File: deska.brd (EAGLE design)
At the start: 50.5 x 49.5 mm, 7 parts

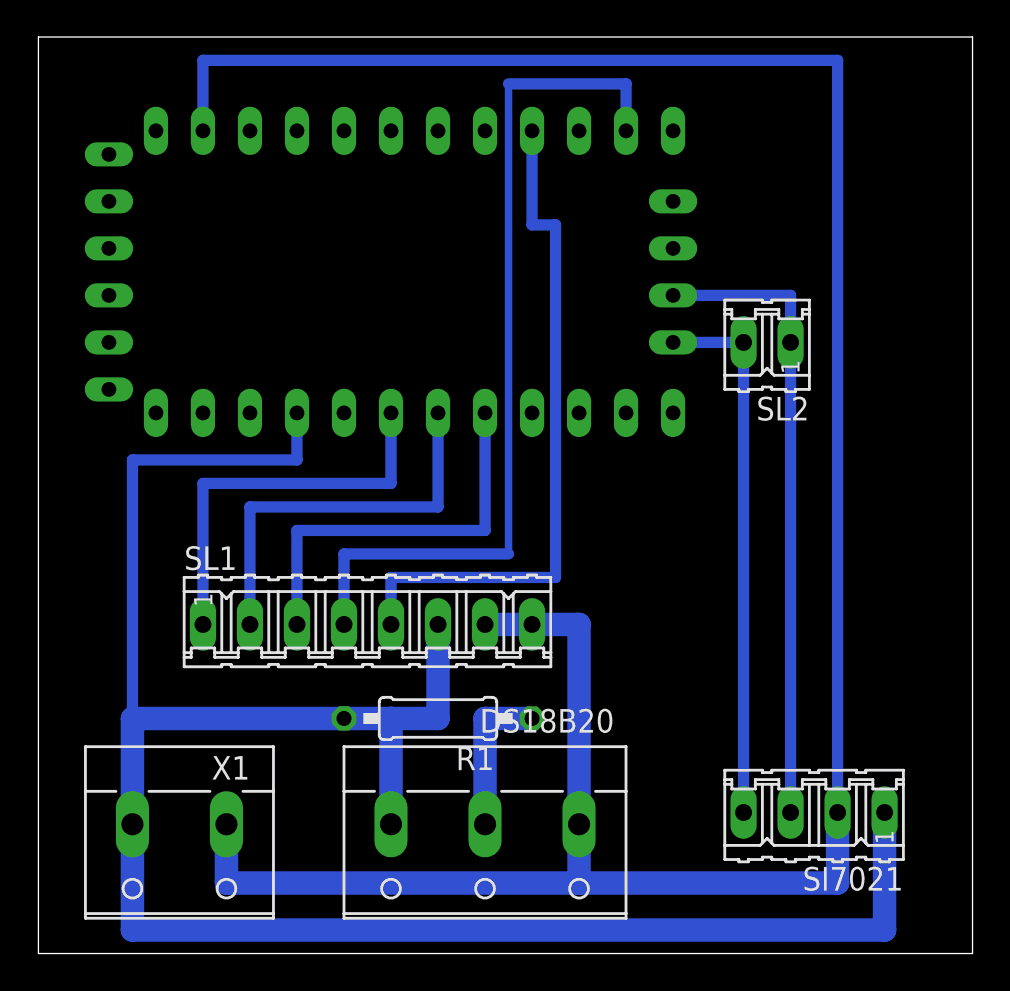
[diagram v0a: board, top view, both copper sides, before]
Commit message: +deska +ino
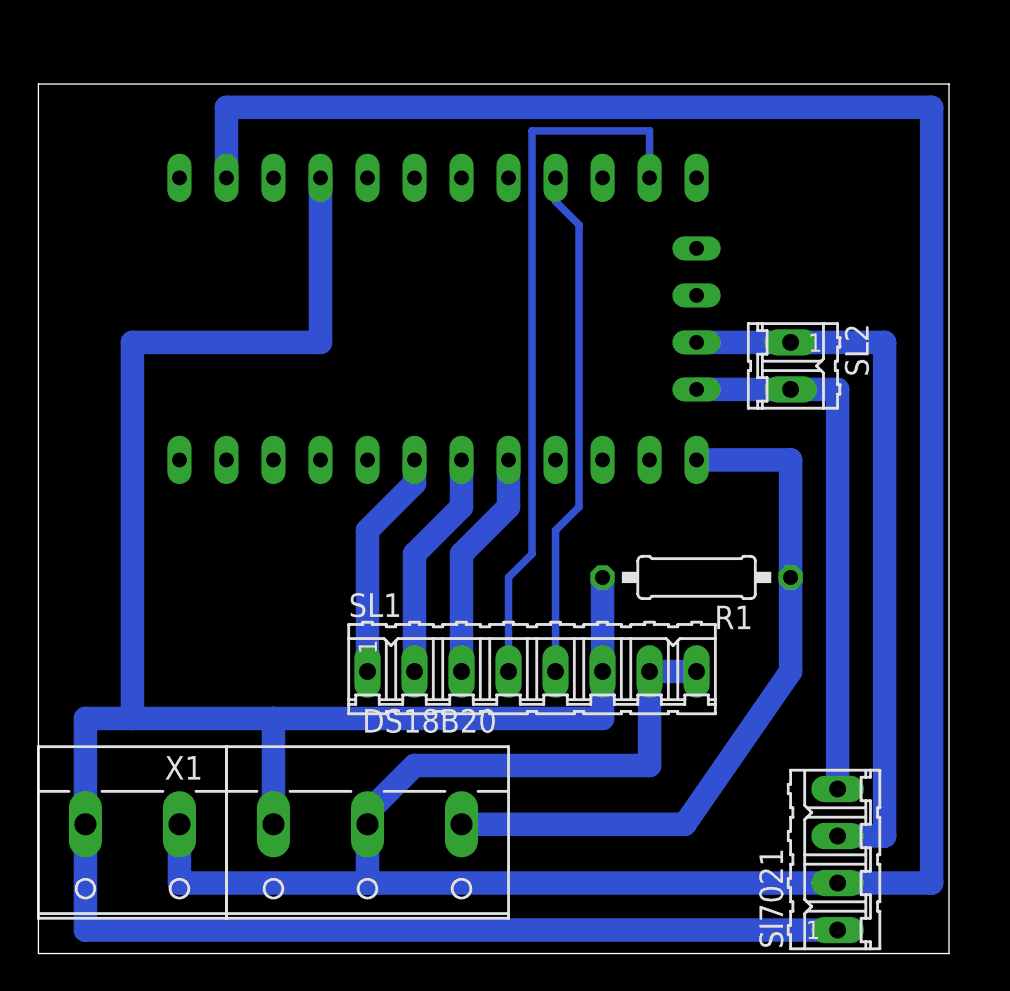
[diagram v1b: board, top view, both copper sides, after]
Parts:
- moved R1 15.9 mm to (35.6, 20.3)
- moved SL1 9.25 mm to (26.7, 15.2)
- moved DS18B20 6.35 mm to (17.8, 6.35)
- moved SI7021 2.84 mm to (43.2, 5.08), turned to 90 degrees
- moved U$1 2.84 mm to (34.3, 33.0)
- moved X1 2.54 mm to (5.08, 6.35)
- moved SL2 1.80 mm to (40.6, 31.8), turned to 270 degrees
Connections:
- net +5V: now also U$1.VCC; no longer U$1.GND1
- net GND: now also DS18B20.2; no longer DS18B20.1
- net N$8: now also DS18B20.1, U$1.D9; no longer DS18B20.2
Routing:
- net N$8: track 8.26 -> 38.6 mm
- net +5V: track 111.1 -> 132.7 mm
- net GND: track 137.8 -> 155.4 mm
- net CLK: track 36.8 -> 27.7 mm
- net RESET: track 21.6 -> 12.5 mm
- net CE: track 21.6 -> 12.5 mm
- net DC: track 21.6 -> 12.5 mm
- net DIN: track 47.0 -> 38.6 mm
- net SCL: track 34.3 -> 39.4 mm
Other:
- board size 50.5 x 49.5 mm -> 49.2 x 47 mm
